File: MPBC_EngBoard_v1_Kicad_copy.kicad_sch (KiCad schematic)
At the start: 4 parts, among them Q1 NMOS, Q2 NMOS, U2 MP1909

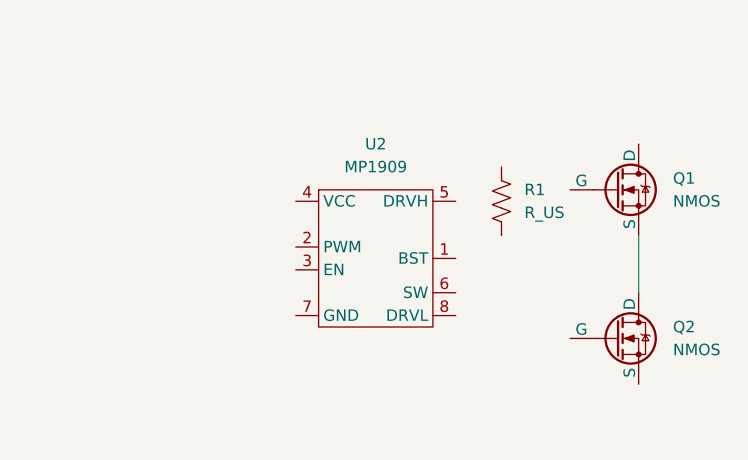
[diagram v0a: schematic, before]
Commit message: Gate Driver Circuit Progress (commit test)
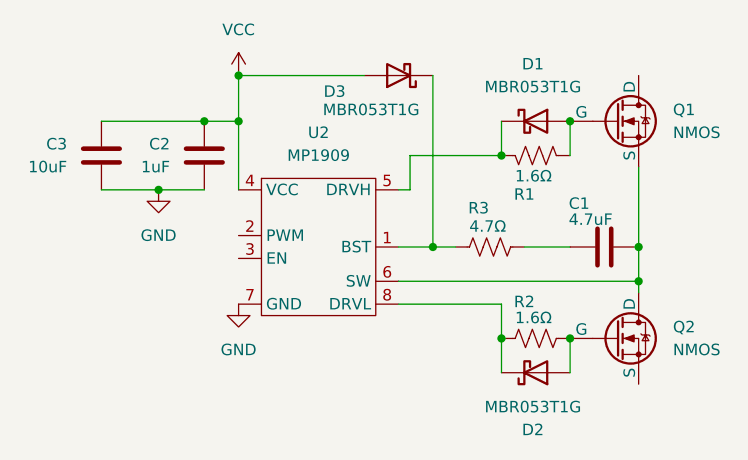
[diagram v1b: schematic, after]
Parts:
- added C1: 4.7uF, symbol Device:C
- added C2: 1uF, symbol Device:C
- added C3: 10uF, symbol Device:C
- added D1, D2, D3: MBR053T1G, symbol Device:D_Schottky
- added R2: 1.6Ω, symbol Device:R_US
- added R3: 4.7Ω, symbol Device:R_US
- R1: value R_US -> 1.6Ω
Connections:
- net at Q1.2 (G): now also R1.1, D1.2 (A)
- net at Q1.3 (S), Q2.1 (D): now also U2.6 (SW), C1.2
- net at R1.2: now also U2.5 (DRVH), D1.1 (K)
- net at Q2.2 (G): now also D2.2 (A), R2.1
- net at U2.1 (BST): now also D3.1 (K), R3.2
- net VCC: now reaches U2.4 (VCC)
- net VCC: now also C2.1, C3.1, D3.2 (A)
- net GND: now reaches U2.7 (GND)
- net GND: now also C2.2, C3.2
- net at U2.8 (DRVL): now also D2.1 (K), R2.2
- new net: C1.1, R3.1
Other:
- title: (none) -> Buck Converter Channel
- moved on the sheet: Q1, R1, U2
